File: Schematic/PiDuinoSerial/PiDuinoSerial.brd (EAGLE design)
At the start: 48.6 x 49.4 mm, 14 parts, among them IC1 ATMEGA8, J1 D0..D7, J2 Analogs, J3 D8_D13, Q1 16Mhz

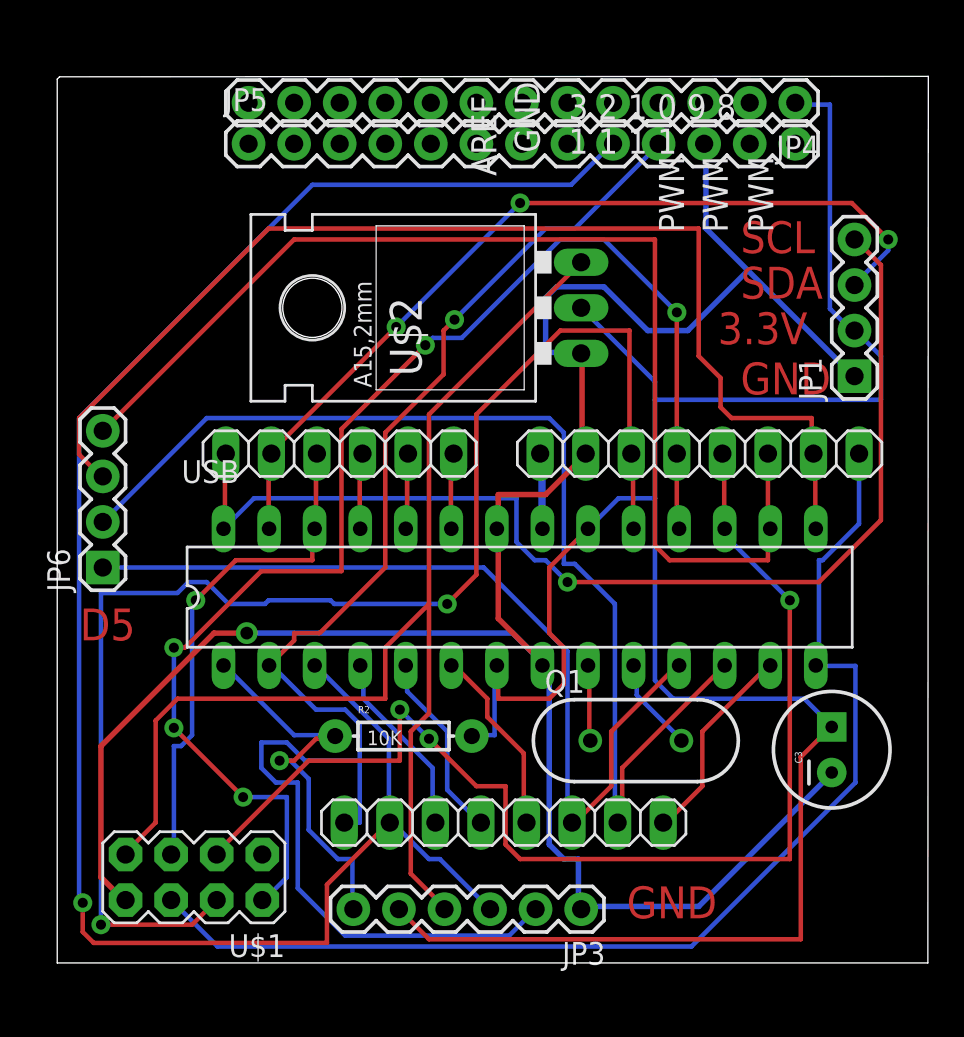
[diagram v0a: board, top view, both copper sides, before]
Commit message: V0.05
Added Android java source code
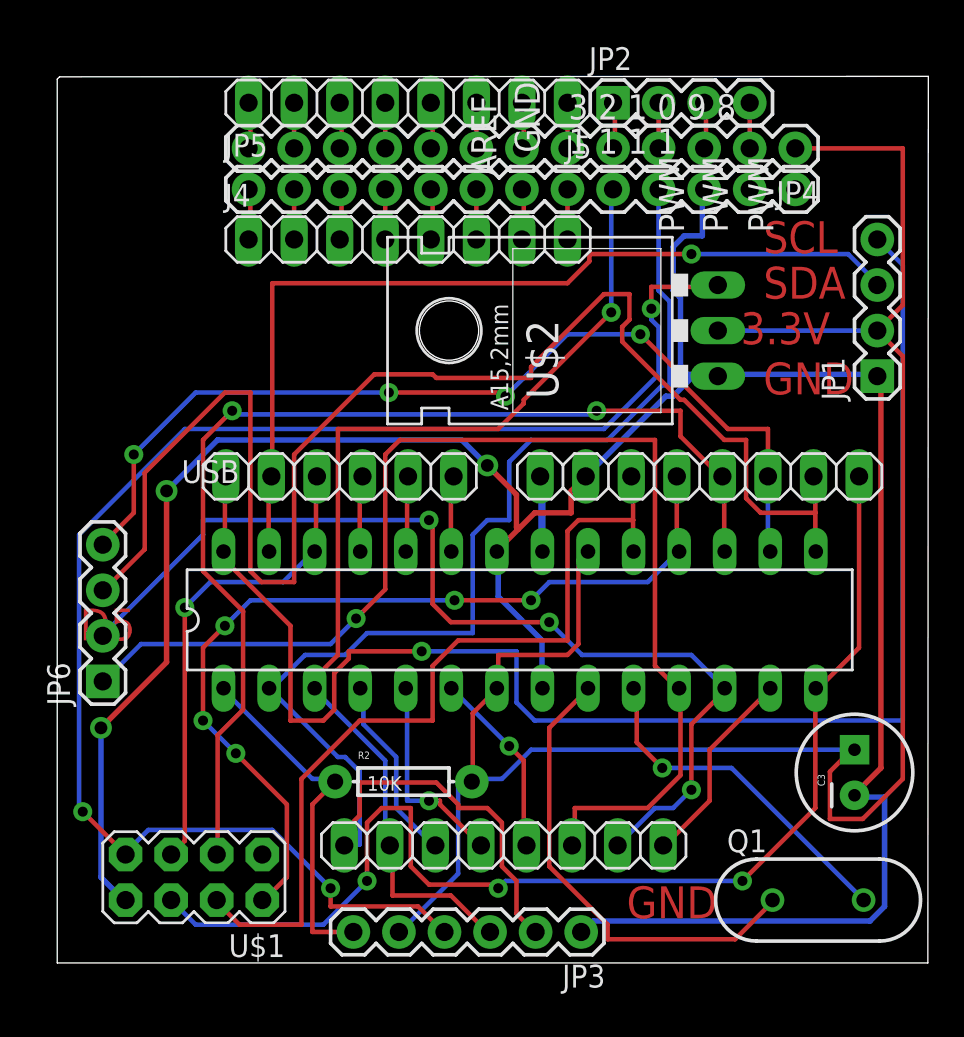
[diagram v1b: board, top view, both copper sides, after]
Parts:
- added J4: PIPins8b, pinhead:1X08
- added J5: PiPins8a, pinhead:1X08
- added JP2: Pi4Pins, SparkFun-Connectors:1X04
- moved Q1 13.5 mm to (42.4, 3.81)
- moved U$2 7.73 mm to (33.0, 35.6)
- moved JP6 6.35 mm to (2.54, 16.0)
- moved R2 2.54 mm to (19.3, 10.4)
- moved JP4 2.54 mm to (41.1, 45.7)
- moved JP5 2.54 mm to (10.7, 43.4)
- moved C3 1.80 mm to (44.5, 10.9)
- moved J2 1.27 mm to (15.7, 27.4)
- moved J3 1.27 mm to (35.8, 27.4)
- moved J1 1.27 mm to (24.9, 6.86)
- moved JP3 1.27 mm to (29.2, 2.03)
- moved IC1 1.27 mm to (25.8, 19.4)
- moved JP1 1.27 mm to (45.7, 33.0)
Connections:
- new net N$10: J4.8, JP5.8
- new net N$11: J5.1, JP4.6
- new net N$12: J5.2, JP4.7
- new net N$13: J5.3, JP4.8
- new net N$14: J5.4, JP4.9
- new net N$15: J5.5, JP4.10
- new net N$16: J5.6, JP4.11
- new net N$17: J5.7, JP4.12
- new net N$18: J5.8, JP4.13
- new net N$19: JP2.1, JP4.5
- new net N$20: JP2.2, JP4.4
- new net N$21: JP2.3, JP4.3
- new net N$22: JP2.4, JP4.2
- new net N$3: J4.1, JP5.1
- new net N$4: J4.2, JP5.2
- new net N$5: J4.3, JP5.3
- new net N$6: J4.4, JP5.4
- new net N$7: J4.5, JP5.5
- new net N$8: J4.6, JP5.6
- new net N$9: J4.7, JP5.7
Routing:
- net D1: track 105.1 -> 59.7 mm
- net D13: track 78.6 -> 47.6 mm, vias 2 -> 0
- net D12: track 74.7 -> 49.6 mm
- net N$2: track 4.26 -> 26.4 mm
- net SCL: track 62.7 -> 83.1 mm
- net D5: track 49.0 -> 68.9 mm, vias 0 -> 1
- net GND: track 127.2 -> 147.0 mm, vias 1 -> 3
- net D9: track 64.8 -> 81.7 mm
- net VCC: track 68.5 -> 85.2 mm, vias 0 -> 3
- net V3.3: track 126.9 -> 111.1 mm
- net N$1: track 5.37 -> 19.4 mm, vias 0 -> 1
- net D10: track 65.0 -> 53.5 mm, vias 0 -> 4
- net D6: track 63.1 -> 56.2 mm, vias 0 -> 3
- net D0: track 83.2 -> 77.3 mm, vias 1 -> 0
- net D11: track 66.6 -> 61.1 mm, vias 3 -> 2
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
